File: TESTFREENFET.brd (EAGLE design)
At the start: 53.3 x 53.3 mm, 21 parts, among them J1 Digital_0_7, J2 Analog, J3 Digital_8_13

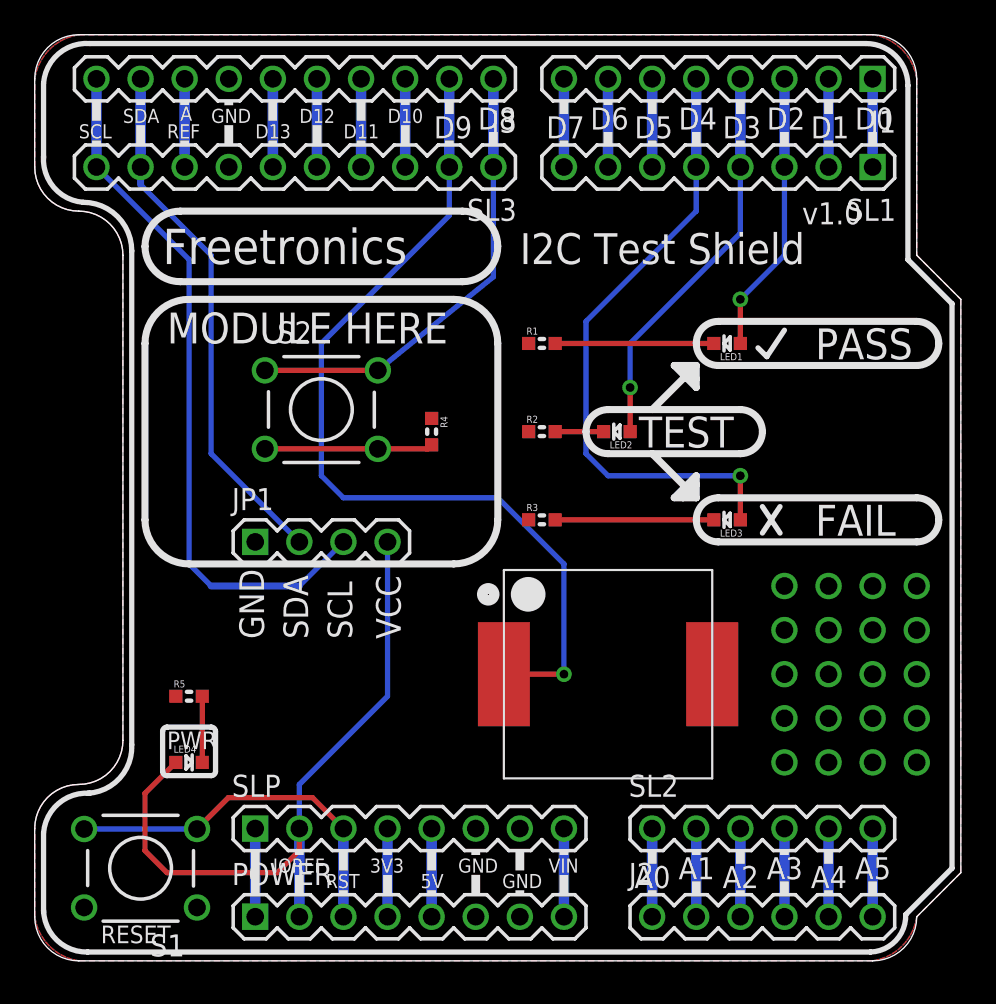
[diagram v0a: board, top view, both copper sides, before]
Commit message: Created TESTFREENFET project for release v1.0
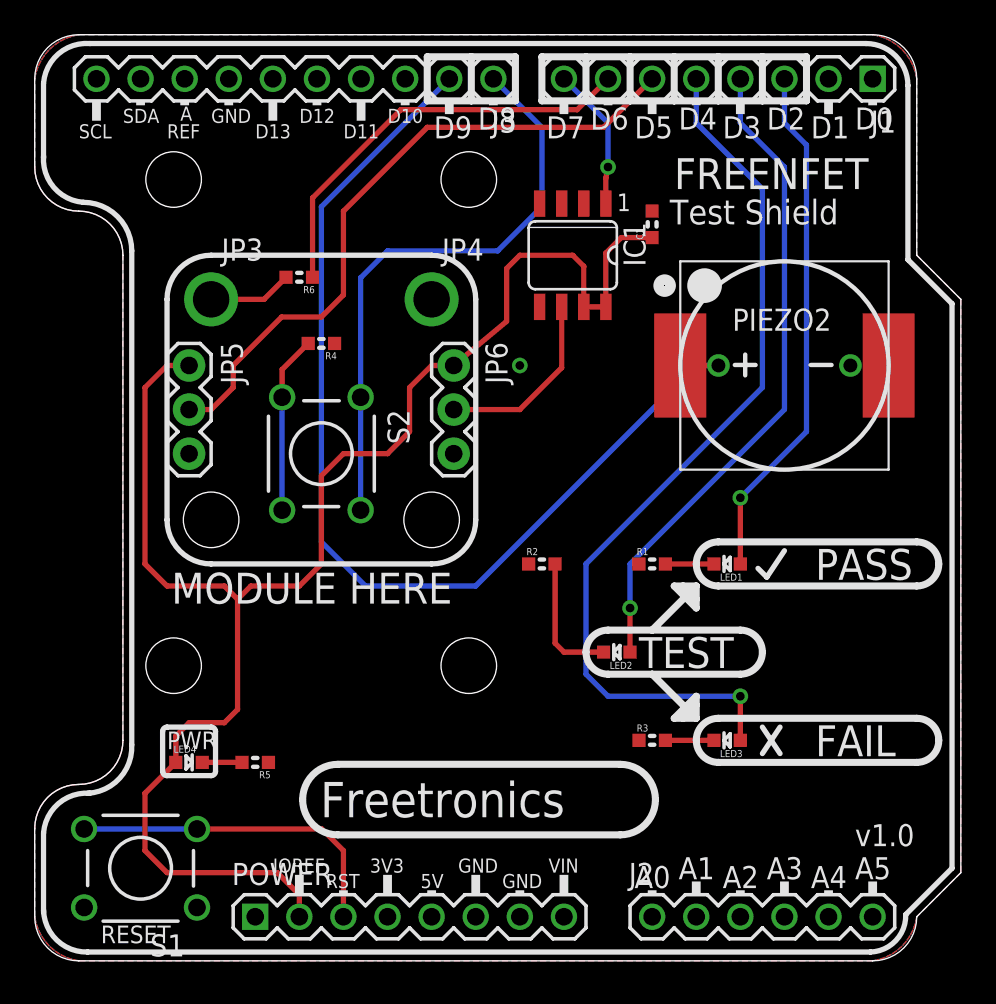
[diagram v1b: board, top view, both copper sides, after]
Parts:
- removed JP1: MODULE, freetronics-master-v1.1:1X04
- removed SL1: Digital_0_7, freetronics:1X08
- removed SL2: Analog, freetronics:1X06
- removed SL3: Digital_8_13, freetronics-original:1X10
- removed SLP: Power, freetronics:1X08
- added C1: 1uF 0603, freetronics-master-v1:0603
- added IC1: WS2811-SOP8, freetronics-jon:SO08-SKINNYPADS
- added JP3: DRAIN, freetronics-jon:1X01_2_1_MM
- added JP4: SOURCE, freetronics-jon:1X01_2_1_MM
- added JP5: IN, freetronics-jon:1X03
- added JP6: OUT, freetronics-jon:1X03
- added PIEZO2: PIEZOPOLARISED, freetronics-jon:PIEZO12MMWIDEPOLARISED
- added R6: 1K, freetronics-jon:0603
- R1, R2, R3: value 560R 0603 -> 560R
- R4: value 1K 0603 -> 1K
- R5: value 1K5 0603 -> 1K5
- moved PIEZO 20.5 mm to (43.2, 34.3)
- moved R1 14.2 mm to (35.6, 22.9)
- moved R3 14.2 mm to (35.6, 12.7)
- moved LED1 12.7 mm to (39.9, 22.9)
- moved LED2 12.7 mm to (33.5, 17.8)
- moved LED3 12.7 mm to (39.9, 12.7)
- moved R4 8.13 mm to (16.5, 35.6), turned to 180 degrees
- moved R2 7.62 mm to (29.2, 22.9)
- moved R5 5.39 mm to (12.7, 11.4), turned to 180 degrees
- moved S2 2.54 mm to (16.5, 29.2), turned to 270 degrees
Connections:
- new net DIN: IC1.6, JP6.2
- new net N$5: JP3.1, R6.2
- new net OUT2: IC1.2
- new net OUT3: IC1.3
- net 3V3: no longer SLP.4
- net 5V: no longer SLP.5
- net A0: no longer SL2.1
- net A1: no longer SL2.2
- net A2: no longer SL2.3
- net A3: no longer SL2.4
- net A4: no longer SL2.5
- net A5: no longer SL2.6
- net AREF: no longer SL3.8
- net D0_RX: no longer SL1.1
- net D10: no longer SL3.3
- net D11_MOSI: no longer SL3.4
- net D12_MISO: no longer SL3.5
- net D13_SCK: no longer SL3.6
- net D1_TX: no longer SL1.2
- net D2: no longer SL1.3
- net D3: no longer SL1.4
- net D4: no longer SL1.5
- net D5: now also JP5.2; no longer SL1.6
- net D6: now also R6.1; no longer SL1.7
- net D7: now also IC1.1; no longer SL1.8
- net D8: no longer SL3.1
- net D9: now also PIEZO2.1; no longer SL3.2
- net GND: now also C1.2, IC1.4, JP4.1, JP5.3, JP6.3, PIEZO2.2; no longer JP1.1, SL3.7, SLP.6, SLP.7
- net IOREF: now also C1.1, IC1.7, IC1.8, JP5.1, JP6.1; no longer JP1.4, SLP.2
- net NC: no longer SLP.1
- net RESET: no longer SLP.3
- net SCL: no longer JP1.3, SL3.10
- net SDA: no longer JP1.2, SL3.9
- net VIN: no longer SLP.8
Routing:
- net IOREF: track 40.7 -> 92.8 mm
- net SCL: track 40.6 -> 0.00 mm
- net D5: track 5.08 -> 38.1 mm
- net SDA: track 30.5 -> 0.00 mm
- net D6: track 5.08 -> 24.4 mm
- net D4: track 36.2 -> 52.0 mm
- net D3: track 23.0 -> 37.8 mm
- net D2: track 16.3 -> 30.0 mm
- net DIN: track 0.00 -> 10.7 mm
- net D9: track 51.8 -> 61.1 mm, vias 1 -> 0
- net D8: track 26.5 -> 34.0 mm
- net N$3: track 9.14 -> 2.79 mm
- net N$1: track 9.14 -> 2.79 mm
- net VIN: track 5.08 -> 0.00 mm
- net NC: track 5.08 -> 0.00 mm
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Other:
- board text added: "(c) 2017 Freetronics Pty Ltd"
- board text added: "1"
- board text added: "D2: GREEN (PASS) D3: YELLOW (BEGIN) D4: RED (FAIL) D5: TESTDATA D6: TESTSENSE D7: OUTPUTSENSE D8: DETECT D9: PIEZO"
- board text added: "FREENFET"
- board text added: "K"
- board text added: "Test Shield"
- board text added: "www.freetronics.com.au"
- board text removed: "(c) 2014 Freetronics Pty Ltd"
- board text removed: "D2: PASS D3: TEST D4: FAIL D8: nDETECT D9: PIEZO"
- board text removed: "I2C Test Shield"
- board text removed: "VCC"
- board text removed: "www.freetronics.com"
